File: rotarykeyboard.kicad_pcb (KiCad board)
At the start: 2 copper layers, 53 parts, among them J101 Breakout, J102 Cortex Debug, J301 USB_C_Receptacle_USB2.0, SW101 RotaryEncoder, SW102 KBPush, SW103 RESET, U101 ATSAMDA1E14B-ABT, U201 QS6K1FRATR, U202 LTP-3784E, U203 PCA9685PW, U301 FTZU6.2ET148, U302 XC9265A331MR-G

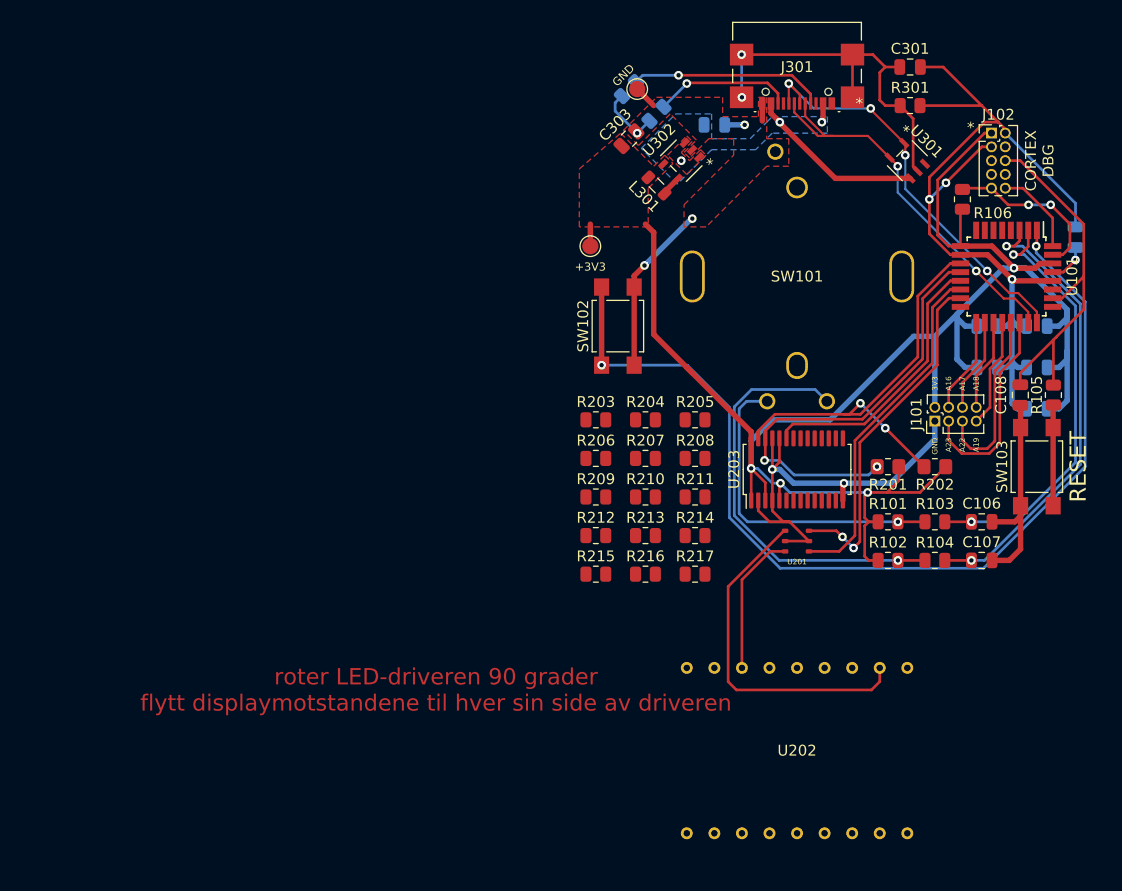
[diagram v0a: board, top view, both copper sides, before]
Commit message: finish routing(?)
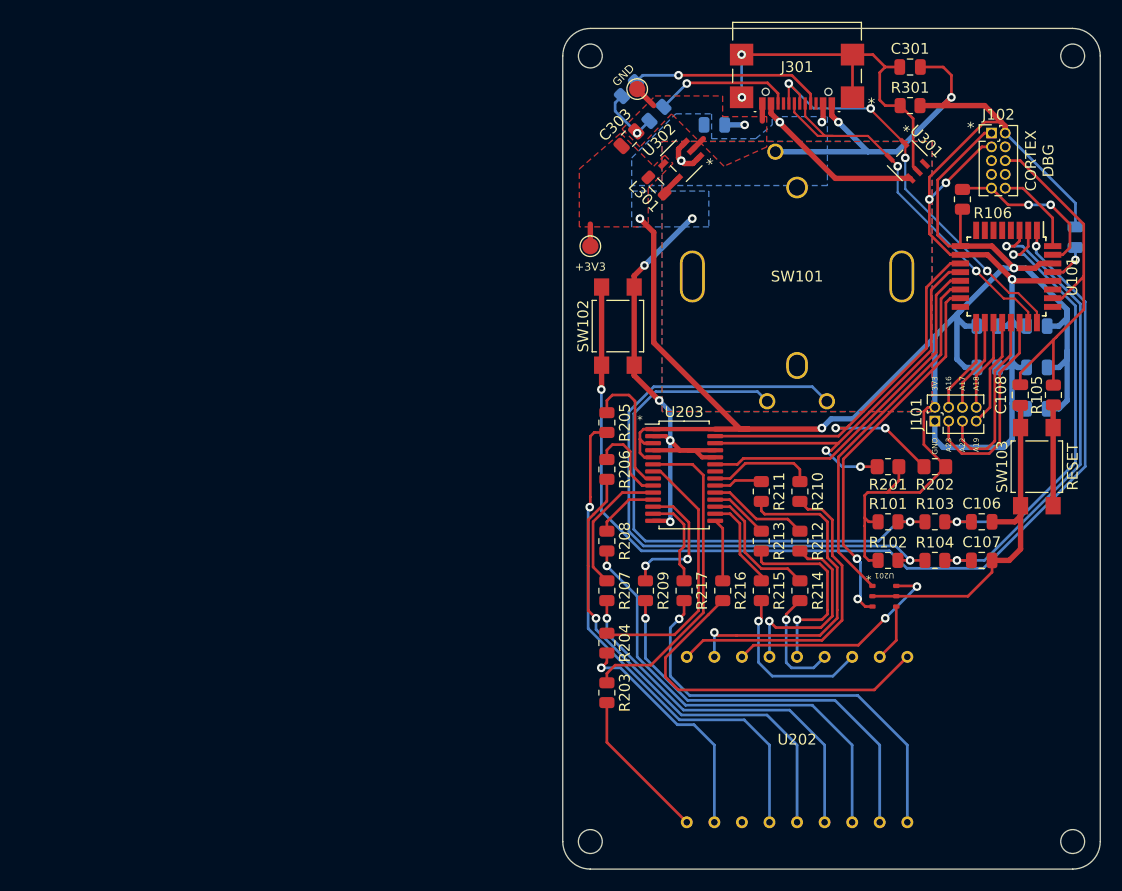
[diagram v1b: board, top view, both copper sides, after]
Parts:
- added REF**: MountingHole_2.2mm_M2_ISO7380, MountingHole:MountingHole_2.2mm_M2_ISO7380, F.Cu at (106.7, 40.6)
- added REF**: MountingHole_2.2mm_M2_ISO7380, MountingHole:MountingHole_2.2mm_M2_ISO7380, F.Cu at (106.7, 113.0)
- added REF**: MountingHole_2.2mm_M2_ISO7380, MountingHole:MountingHole_2.2mm_M2_ISO7380, F.Cu at (62.2, 40.6)
- added REF**: MountingHole_2.2mm_M2_ISO7380, MountingHole:MountingHole_2.2mm_M2_ISO7380, F.Cu at (62.2, 113.0)
- moved R203 25.2 mm to (63.8, 99.3), turned to -90 degrees
- moved R204 20.9 mm to (63.8, 94.7), turned to -90 degrees
- moved R212 18.8 mm to (81.5, 85.3), turned to -90 degrees
- moved R215 15.3 mm to (78.0, 89.9), turned to -90 degrees
- moved R210 14.2 mm to (81.5, 80.8), turned to -90 degrees
- moved R207 12.7 mm to (63.8, 89.9), turned to -90 degrees
- moved R208 11.1 mm to (63.8, 85.3), turned to -90 degrees
- moved R214 10.9 mm to (81.5, 89.9), turned to -90 degrees
- moved R213 10.7 mm to (78.0, 85.3), turned to -90 degrees
- moved U203 10.4 mm to (70.9, 79.2), turned to 0 degrees
- moved R209 9.77 mm to (67.3, 89.9), turned to -90 degrees
- moved U201 9.51 mm to (89.3, 90.4), turned to -90 degrees
- moved R205 8.13 mm to (63.8, 74.4), turned to -90 degrees
- moved R216 7.28 mm to (74.4, 89.9), turned to -90 degrees
- moved R211 6.13 mm to (78.0, 80.8), turned to -90 degrees
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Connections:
- R203 pad 1: Net-(R203-Pad1) -> Net-(U203-Pad6)
- R203 pad 2: Net-(R203-Pad2) -> Net-(U202-Pad1)
- R204 pad 1: Net-(R204-Pad1) -> Net-(U203-Pad7)
- R204 pad 2: Net-(R204-Pad2) -> Net-(U202-Pad2)
- R205 pad 1: Net-(R205-Pad1) -> Net-(U203-Pad8)
- R206 pad 1: Net-(R206-Pad1) -> Net-(U203-Pad9)
- R206 pad 2: Net-(R206-Pad2) -> Net-(U202-Pad5)
- R207 pad 1: Net-(R207-Pad1) -> Net-(U203-Pad10)
- R207 pad 2: Net-(R207-Pad2) -> Net-(U202-Pad6)
- R208 pad 1: Net-(R208-Pad1) -> Net-(U203-Pad11)
- R209 pad 1: Net-(R209-Pad1) -> Net-(U203-Pad12)
- U202 pad 1: Net-(R203-Pad1) -> Net-(U202-Pad1)
- U202 pad 2: Net-(R204-Pad1) -> Net-(U202-Pad2)
- U202 pad 4: Net-(R205-Pad1) -> Net-(R205-Pad2)
- U202 pad 5: Net-(R206-Pad1) -> Net-(U202-Pad5)
- U202 pad 6: Net-(R207-Pad1) -> Net-(U202-Pad6)
- U202 pad 7: Net-(R208-Pad1) -> Net-(R208-Pad2)
- U202 pad 8: Net-(R209-Pad1) -> Net-(R209-Pad2)
- U203 pad 10: Net-(R207-Pad2) -> Net-(U203-Pad10)
- U203 pad 11: Net-(R208-Pad2) -> Net-(U203-Pad11)
- U203 pad 12: Net-(R209-Pad2) -> Net-(U203-Pad12)
- U203 pad 6: Net-(R203-Pad2) -> Net-(U203-Pad6)
- U203 pad 7: Net-(R204-Pad2) -> Net-(U203-Pad7)
- U203 pad 8: Net-(R205-Pad2) -> Net-(U203-Pad8)
- U203 pad 9: Net-(R206-Pad2) -> Net-(U203-Pad9)
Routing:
- net Net-(R205-Pad2): track 0.00 -> 47.7 mm, vias 0 -> 1
- net Net-(U202-Pad5): track 0.00 -> 44.9 mm, vias 0 -> 1
- net Net-(R208-Pad2): track 0.00 -> 41.2 mm, vias 0 -> 1
- net GND: track 170.2 -> 211.0 mm, vias 9 -> 12
- net Net-(R217-Pad2): track 0.00 -> 39.1 mm, vias 0 -> 1
- net Net-(R209-Pad2): track 0.00 -> 37.3 mm, vias 0 -> 1
- net Net-(U202-Pad6): track 0.00 -> 34.5 mm, vias 0 -> 1
- net Net-(R216-Pad2): track 0.00 -> 33.3 mm
- net Net-(R211-Pad2): track 0.00 -> 31.0 mm, vias 0 -> 1
- net Net-(U203-Pad6): track 0.00 -> 29.8 mm
- net Net-(R210-Pad2): track 0.00 -> 29.0 mm
- net Net-(U201-Pad4): track 32.0 -> 5.27 mm
- net Net-(U203-Pad7): track 0.00 -> 24.4 mm
- net Net-(R101-Pad2): track 30.0 -> 53.3 mm
- net Net-(U202-Pad2): track 0.00 -> 22.1 mm, vias 0 -> 1
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- added copper zone on B.Cu, net +3V3
- removed copper zone on F.Cu, net +5V
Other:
- board outline added: 49.5 x 77.5 mm
- board text removed: "roter LED-driveren 90 grader flytt displaymotstandene til hver sin side av driveren"
